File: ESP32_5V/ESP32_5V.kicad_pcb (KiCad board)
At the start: 4 copper layers, 90 x 70 mm, 95 parts, among them J1 Barrel_Jack_MountingPin, J10 Conn_01x11, J11 Conn_01x11, J12 Conn_01x11, J13 Conn_01x11, J15 Screw_Terminal_01x11, J16 Screw_Terminal_01x11, J2 Conn_01x11, J3 Conn_01x11, J4 Conn_01x11, J5 Conn_01x11, J6 Conn_01x11, J7 Conn_01x11, J8 Conn_01x11, J9 Conn_01x11, U1 TPS563201, U2 TPS563201, U3 SN74LVC245APW, U4 SN74LVC245APW, U5 SN74LVC245APW

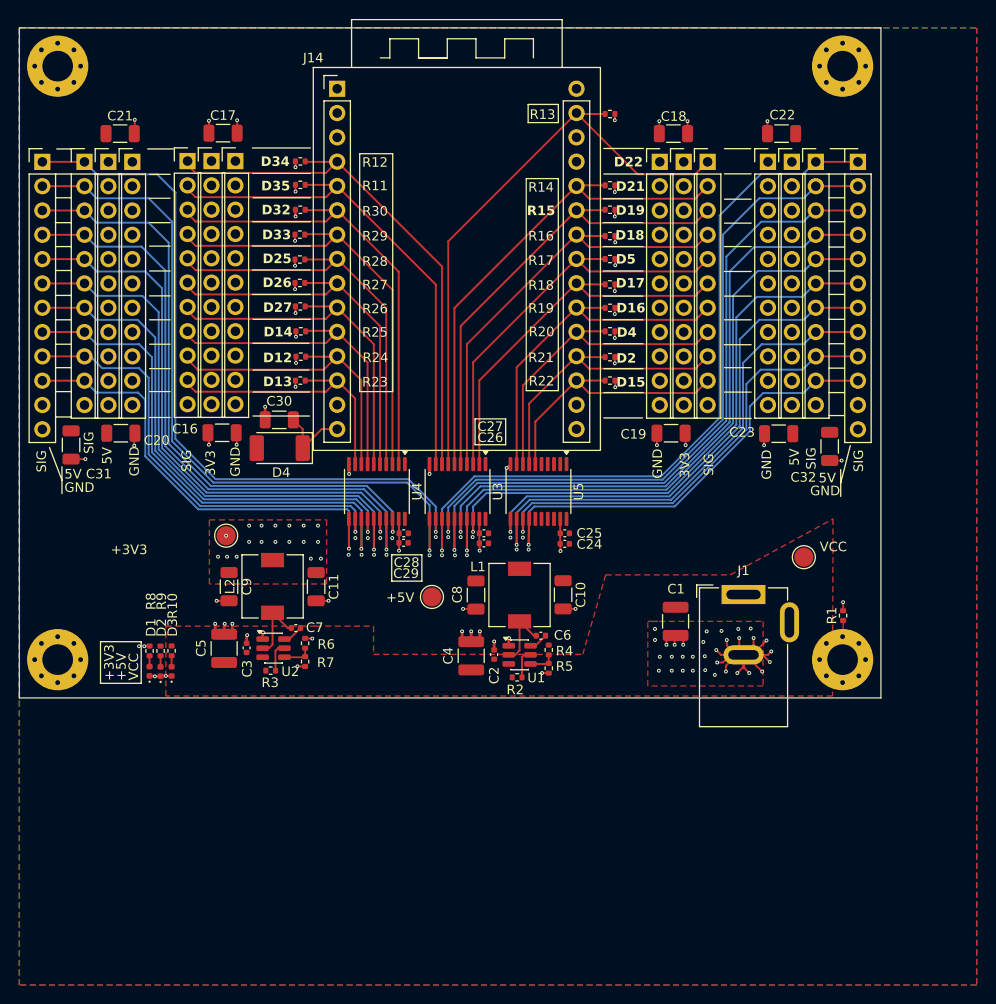
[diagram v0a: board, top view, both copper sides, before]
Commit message: update
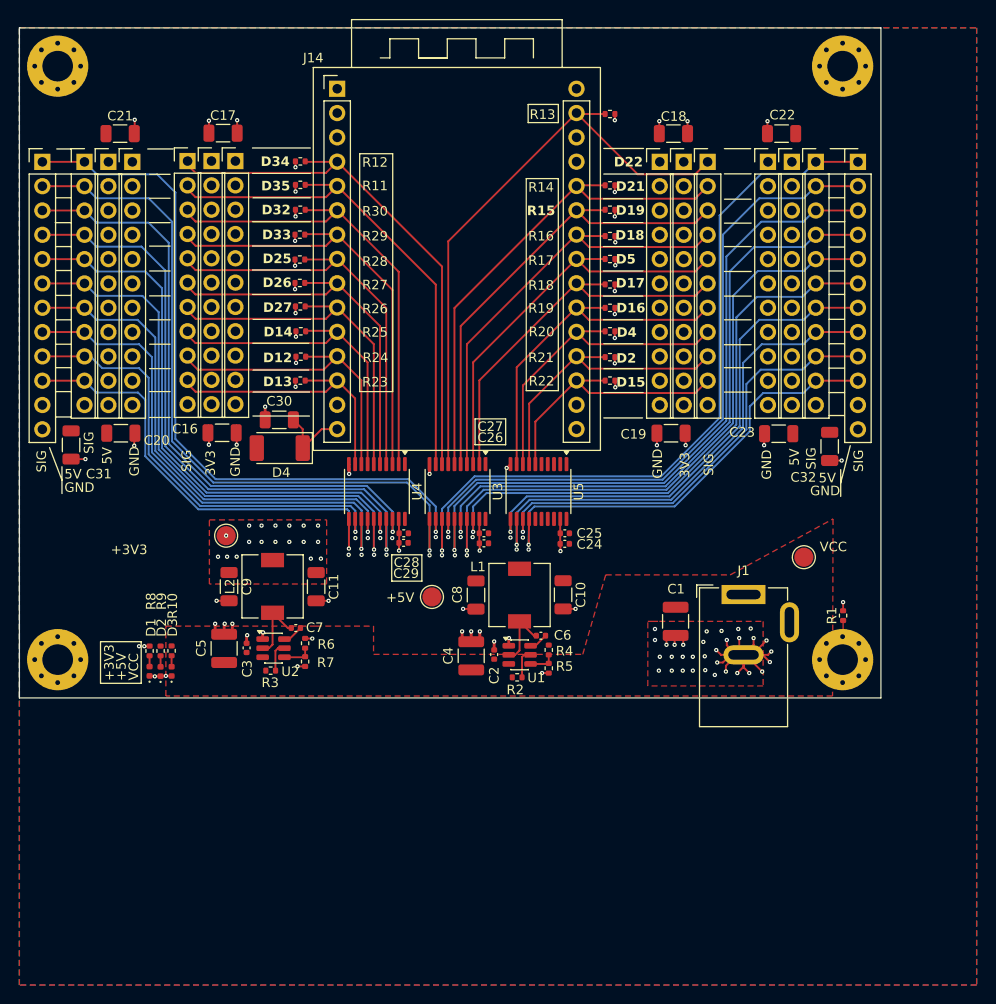
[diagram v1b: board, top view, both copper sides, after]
